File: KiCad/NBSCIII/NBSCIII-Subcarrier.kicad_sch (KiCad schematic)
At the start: 7 parts, among them U4 4011, U5 4029, U6 4029, U7 4027, U8 4027

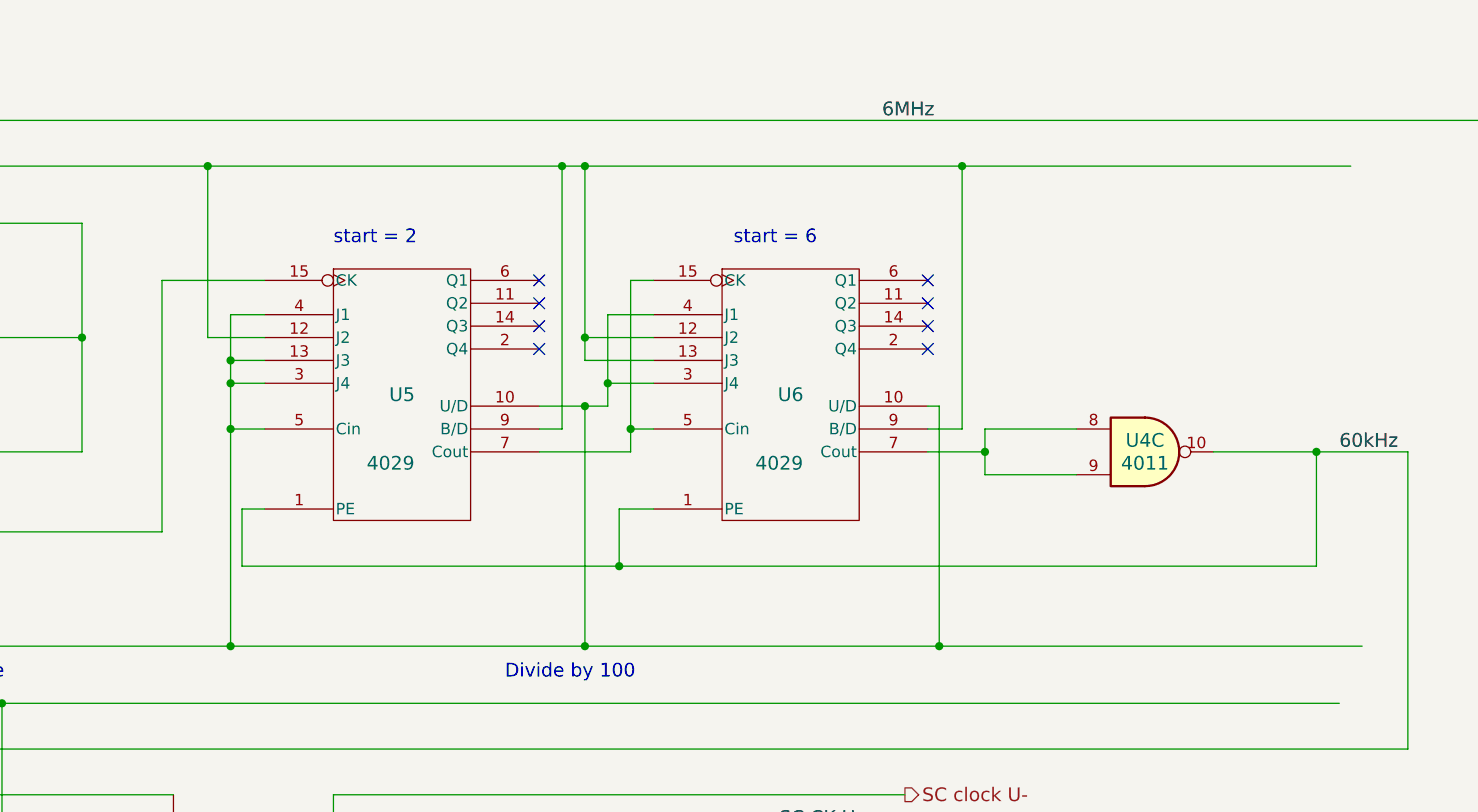
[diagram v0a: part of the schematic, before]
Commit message: unrescue 4029
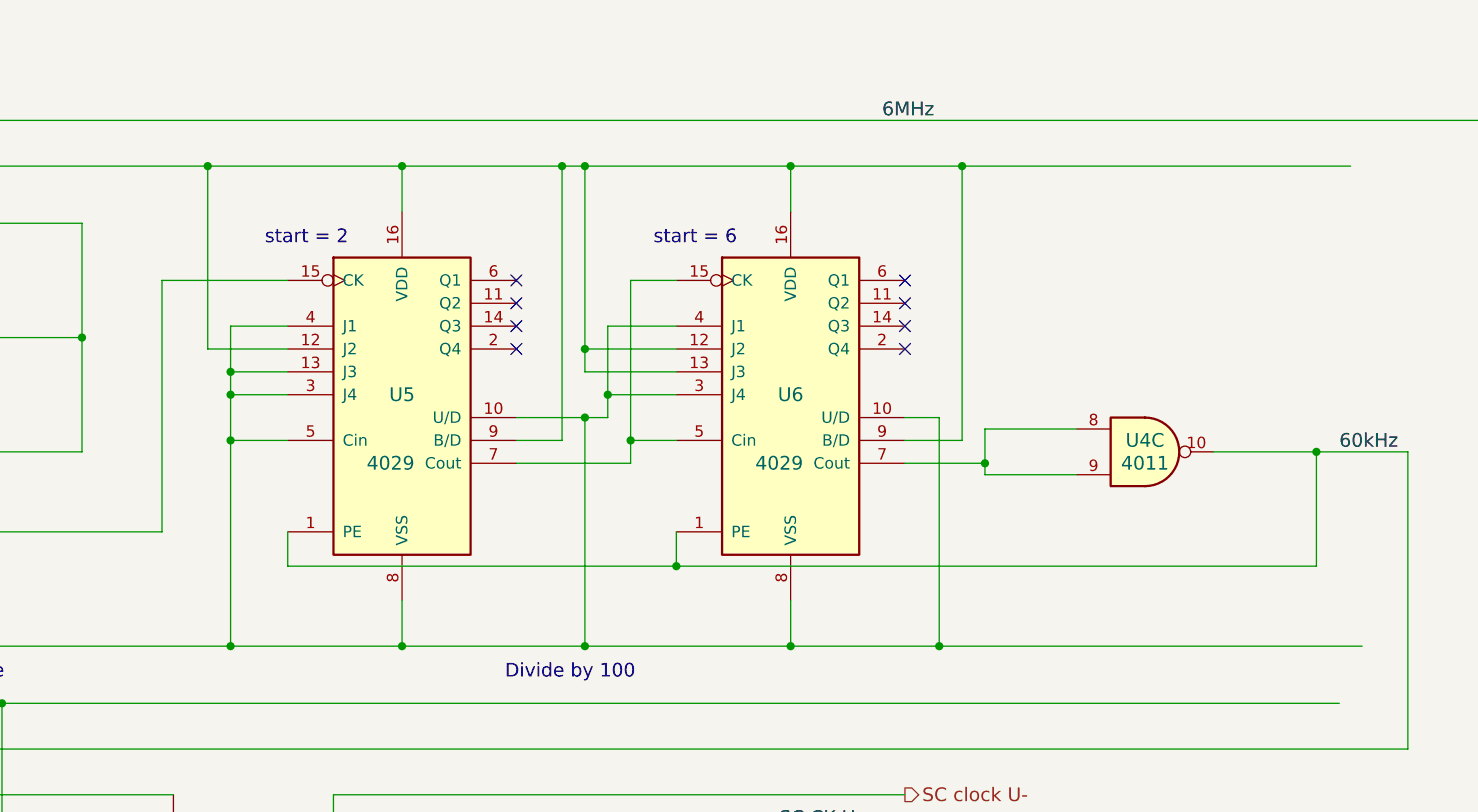
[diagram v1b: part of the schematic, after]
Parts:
- U5, U6: symbol NBSCIII-rescue:4029 -> 4xxx:4029
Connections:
- net +12V: now also U5.16 (VDD), U6.16 (VDD)
- net GND: now also U5.8 (VSS), U6.8 (VSS)
- net VDD: no longer U5.16 (VDD), U6.16 (VDD)
- net VSS: no longer U5.8 (VSS), U6.8 (VSS)

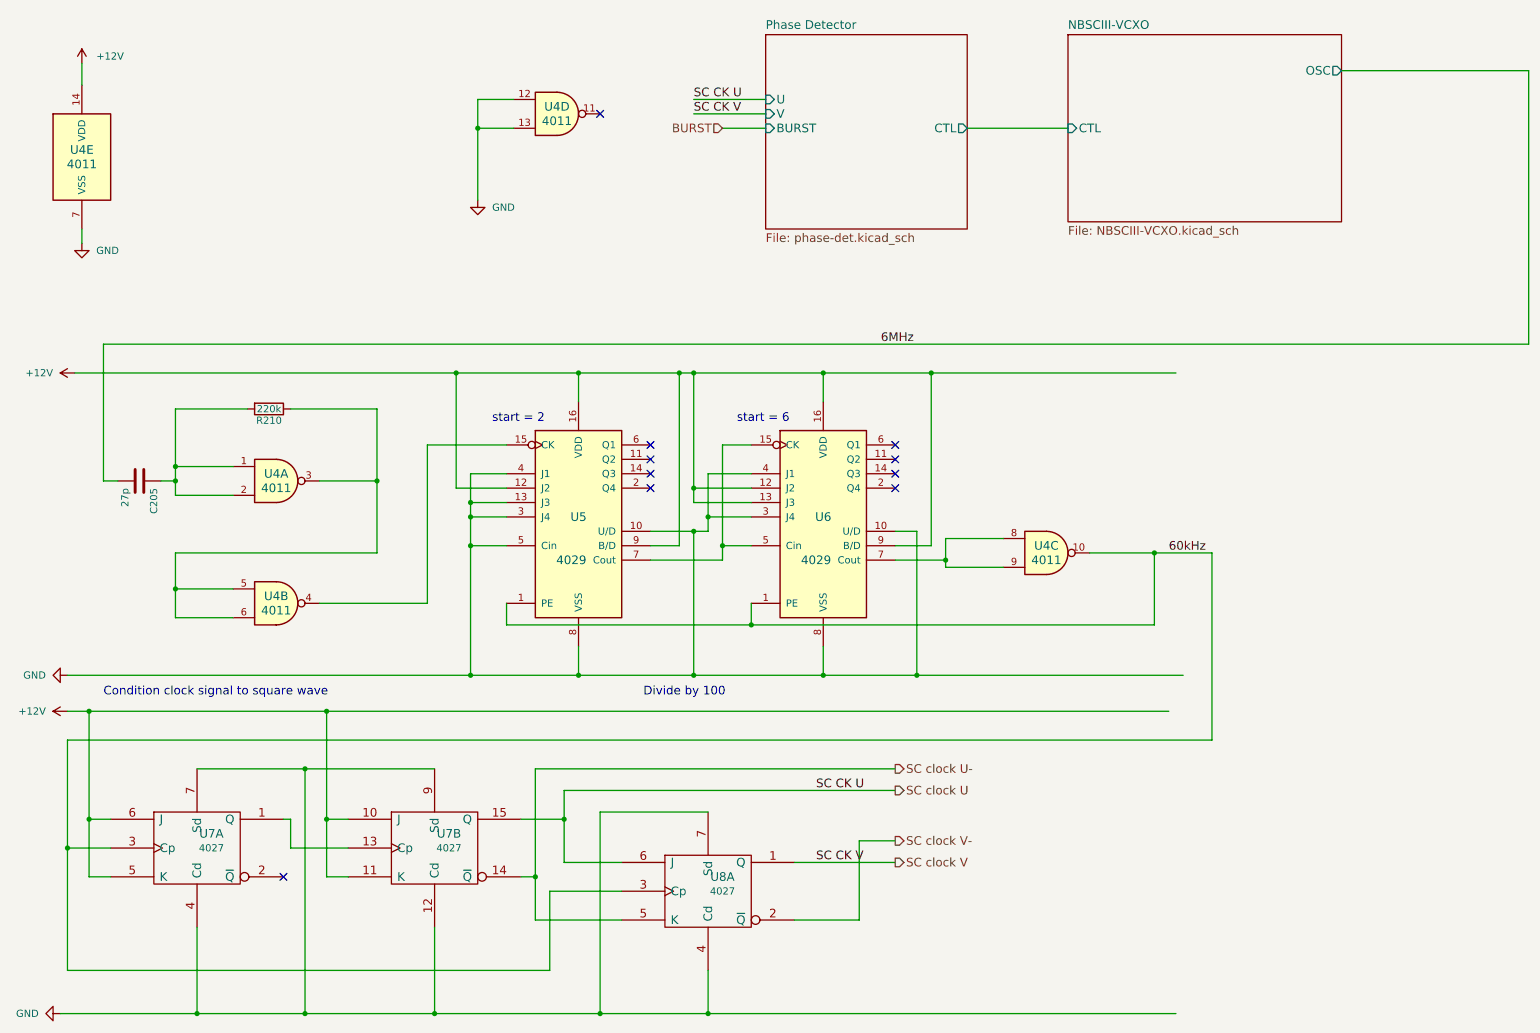
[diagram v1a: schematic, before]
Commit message: derescue 4027
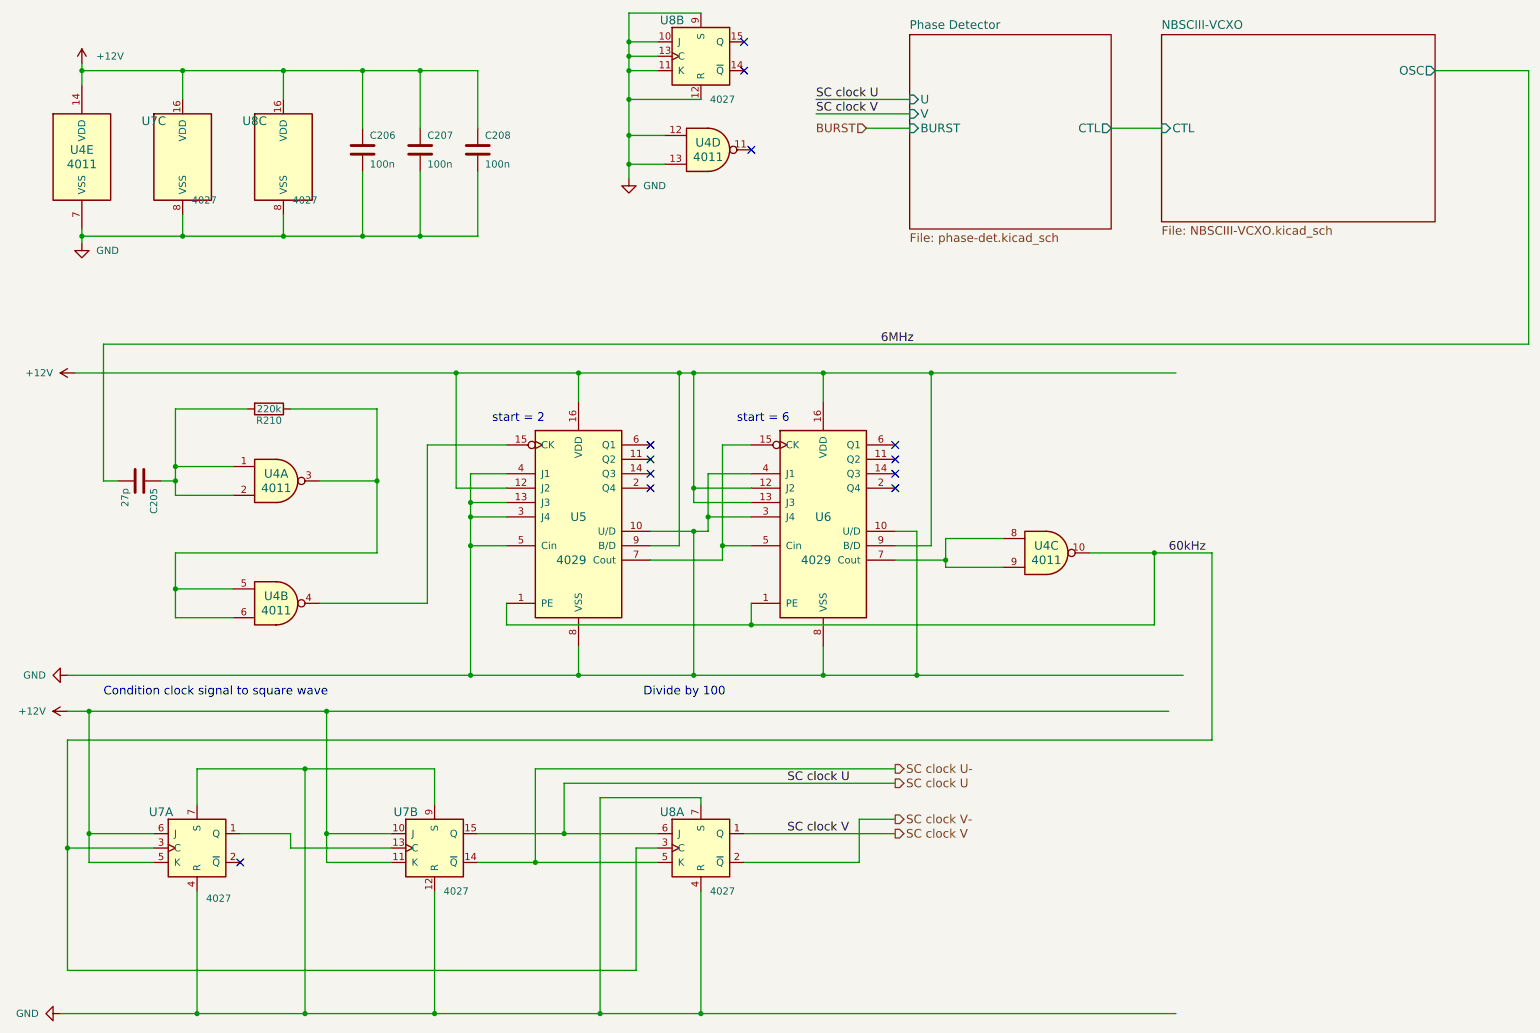
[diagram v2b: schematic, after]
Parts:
- added C206, C207, C208: 100n, symbol Device:C
- added unit 3 of U7
- added unit 3 of U8
- added unit 2 of U8
- U7, U8: symbol NBSCIII-rescue:4027 -> 4xxx:4027
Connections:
- net +12V: now also C206.1, C207.1, C208.1, U7.16 (VDD), U8.16 (VDD)
- net GND: now also C206.2, C207.2, C208.2, U7.8 (VSS), U8.10 (J), U8.11 (K), U8.12 (R), U8.13 (C), U8.8 (VSS), U8.9 (S)
- removed net VDD: U7.16 (VDD), U7.16 (VDD), U8.16 (VDD)
- removed net VSS: U7.8 (VSS), U7.8 (VSS), U8.8 (VSS)
- no-connect marks 10 -> 12
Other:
- moved on the sheet: U4D, U8A
